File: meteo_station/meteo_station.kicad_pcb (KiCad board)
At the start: 2 copper layers, 100 x 87.3 mm, 16 parts, among them SW1 SW_SPDT, U1 TP4056, U2 ESP32-WROOM, U3 DS18B20, U4 BH1750, U5 BME280

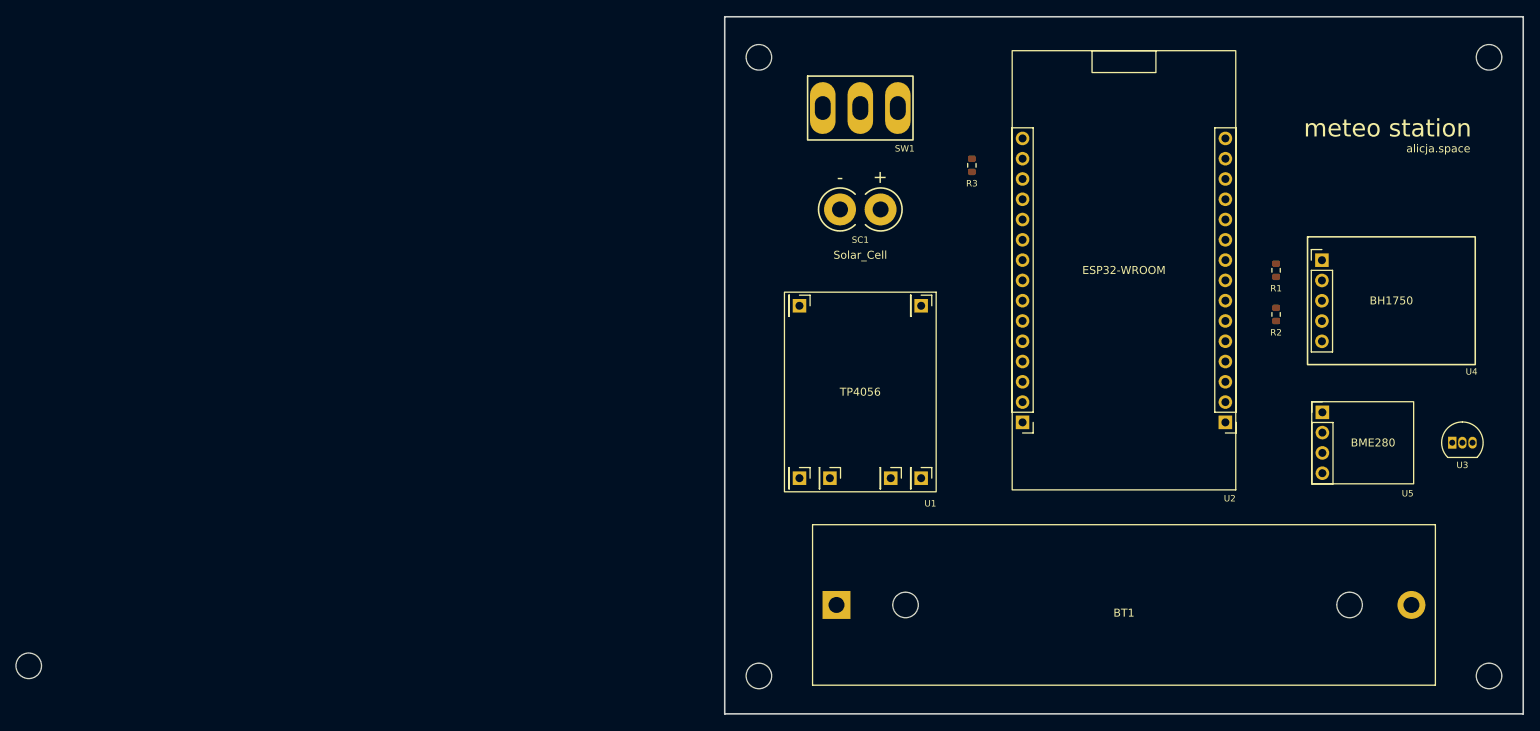
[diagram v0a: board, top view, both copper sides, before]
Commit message: Add some routes
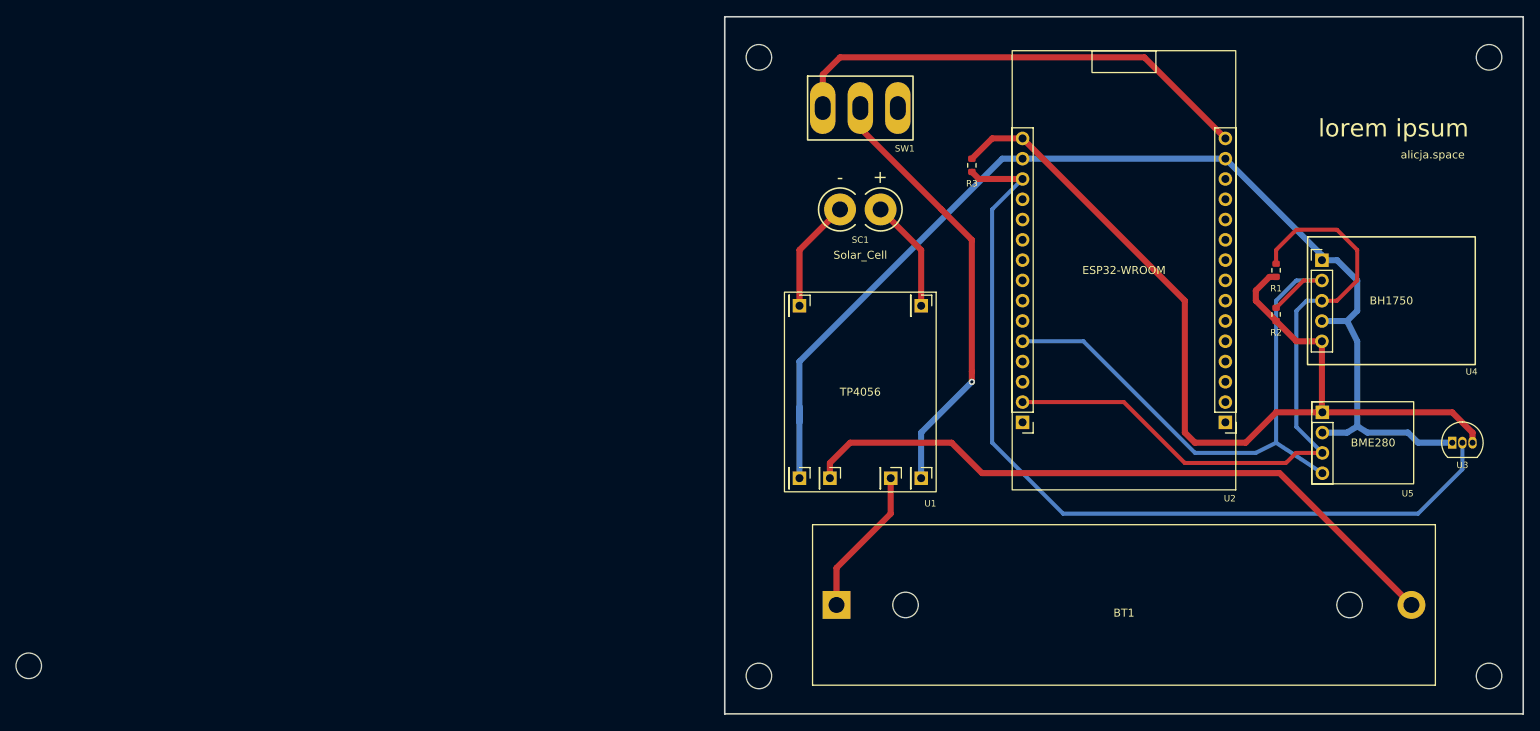
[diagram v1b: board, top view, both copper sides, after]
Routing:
- net GND: track 0.00 -> 143.1 mm
- net 3V3: track 0.00 -> 116.9 mm
- net Net-(R3-Pad2): track 0.00 -> 109.5 mm
- net SCL: track 0.00 -> 87.4 mm
- net Net-(BT1-Pad2): track 0.00 -> 84.2 mm
- net SDA: track 0.00 -> 76.5 mm
- net Net-(SW1-Pad1): track 0.00 -> 59.7 mm
- net Net-(SW1-Pad2): track 0.00 -> 54.8 mm, vias 0 -> 1
- net Net-(BT1-Pad1): track 0.00 -> 18.7 mm
- net Net-(SC1-Pad2): track 0.00 -> 14.2 mm
- net Net-(SC1-Pad1): track 0.00 -> 14.2 mm
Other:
- board text added: "lorem ipsum"
- board text removed: "meteo station"
